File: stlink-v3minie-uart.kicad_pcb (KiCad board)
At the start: 2 copper layers, 10 x 3 mm, 3 parts, among them J1 Conn_01x05, J2 Conn_02x05_Top_Bottom, J3 Conn_01x04_Pin

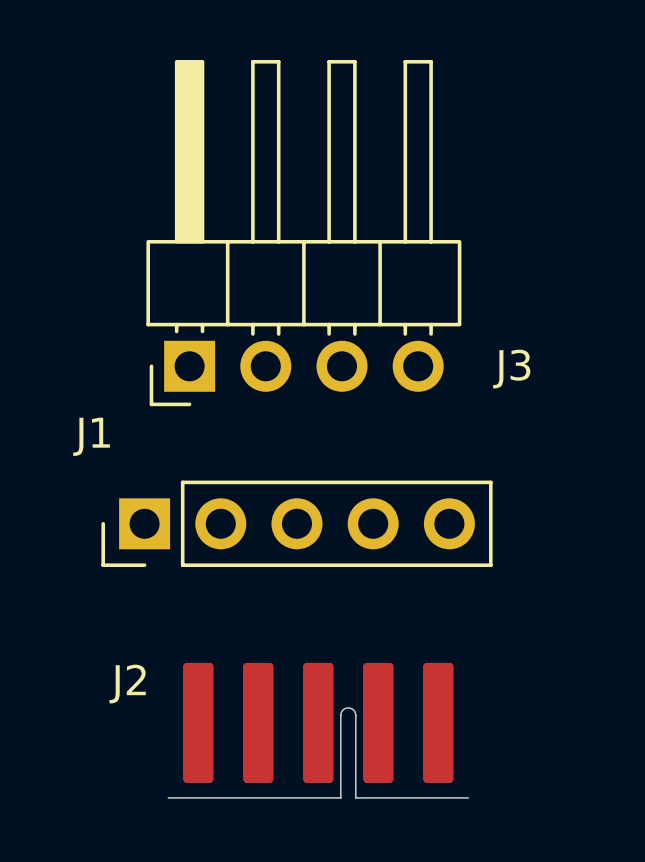
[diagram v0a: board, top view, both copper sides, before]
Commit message: pcb: oui
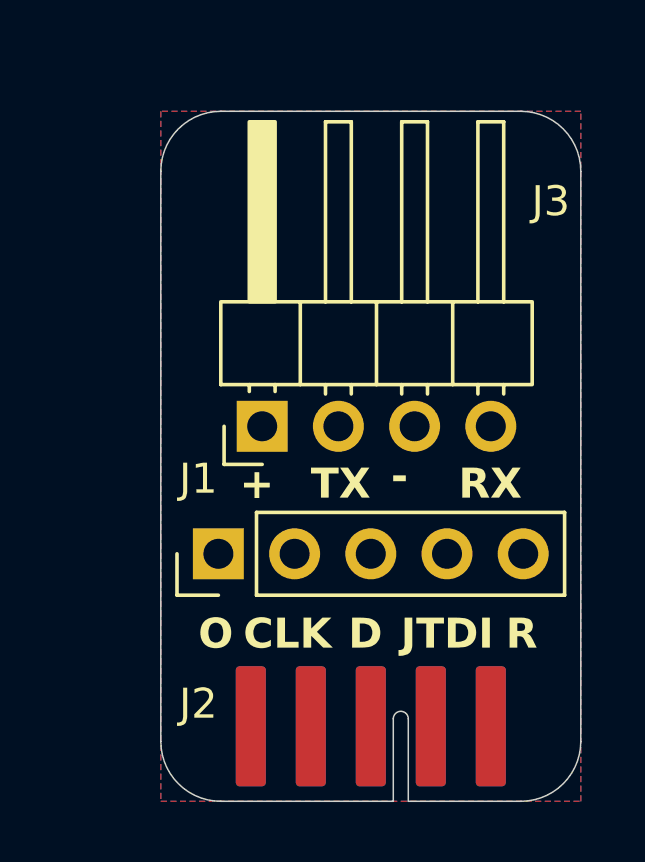
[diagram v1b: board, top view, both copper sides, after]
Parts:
- moved J3 3.14 mm to (146.4, 103.5)
- moved J1 2.66 mm to (144.9, 107.8)
- moved J2 1.75 mm to (147.0, 116.0)
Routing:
- added copper zone on B.Cu, net GND
- added copper zone on F.Cu, net GND
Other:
- board size 10 x 3 mm -> 14 x 23 mm
- board text added: "+"
- board text added: "-"
- board text added: "CLK"
- board text added: "D"
- board text added: "JTDI"
- board text added: "O"
- board text added: "R"
- board text added: "RX"
- board text added: "TX"
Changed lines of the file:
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@@
 	(footprint "GLCS:KYOCERA_AVX9159-006"
 		(layer "F.Cu")
-		(at 145.25 115.8875 180)
+		(at 147 116 180)
 		(descr "board to board 10 pin edge connector https://www.kyocera-avx.com/download/connectors/Conn-Sales-Drawings/9XXX/9159-06X.zip")
 		(tags "edge b2b")
 		(property "Reference" "J2"
-			(at 3.25 3.8875 0)
+			(at 2.75 3.25 0)
 			(layer "F.SilkS")
 			(effects
@@
 	(footprint "Connector_PinHeader_2.54mm:PinHeader_1x05_P2.54mm_Vertical"
 		(layer "F.Cu")
-		(at 142.46 106.75 90)
+		(at 144.92 107.75 90)
 		(descr "Through hole straight pin header, 1x05, 2.54mm pitch, single row")
 		(tags "Through hole pin header THT 1x05 2.54mm single row")
 		(property "Reference" "J1"
-			(at 3 -1.67 180)
+			(at 2.5 -0.67 180)
 			(layer "F.SilkS")
 			(effects
@@
 	(footprint "Connector_PinHeader_2.54mm:PinHeader_1x04_P2.54mm_Horizontal"
 		(layer "F.Cu")
-		(at 143.96 101.5 90)
+		(at 146.38 103.5 90)
 		(descr "Through hole angled pin header, 1x04, 2.54mm pitch, 6mm pin length, single row")
 		(tags "Through hole angled pin header THT 1x04 2.54mm single row")
 		(property "Reference" "J3"
-			(at 0 10.83 180)
+			(at 7.5 9.62 180)
 			(layer "F.SilkS")
 			(effects
@@
 			)
 		)
+	)
+	(gr_arc
+		(start 143 95)
+		(mid 143.585786 93.585786)
+		(end 145 93)
+		(stroke
+			(width 0.05)
+			(type default)
+		)
+		(layer "Edge.Cuts")
+	)
+	(gr_line
+		(start 143 114)
+		(end 143 95)
+		(stroke
+			(width 0.05)
+			(type default)
+		)
+		(layer "Edge.Cuts")
+	)
+	(gr_arc
+		(start 145 116)
+		(mid 143.585786 115.414214)
+		(end 143 114)
+		(stroke
+			(width 0.05)
+			(type default)
+		)
+		(layer "Edge.Cuts")
+	)
+	(gr_line
+		(start 155 93)
+		(end 145 93)
+		(stroke
+			(width 0.05)
+			(type default)
+		)
+		(layer "Edge.Cuts")
+	)
+	(gr_arc
+		(start 155 93)
+		(mid 156.414214 93.585786)
+		(end 157 95)
+		(stroke
+			(width 0.05)
+			(type default)
+		)
+		(layer "Edge.Cuts")
+	)
+	(gr_arc
+		(start 157 114)
+		(mid 156.414214 115.414214)
+		(end 155 116)
+		(stroke
+			(width 0.05)
+			(type default)
+		)
+		(layer "Edge.Cuts")
+	)
+	(gr_line
+		(start 157 114)
+		(end 157 95)
+		(stroke
+			(width 0.05)
+			(type default)
+		)
+		(layer "Edge.Cuts")
+	)
+	(gr_text "O"
+		(at 144.25 111 0)
+		(layer "F.SilkS" knockout)
+		(effects
+			(font
+				(size 1 1)
+				(thickness 0.2)
+				(bold yes)
+			)
+			(justify left bottom)
+		)
+	)
+	(gr_text "+"
+		(at 145.628589 106.012058 0)
+		(layer "F.SilkS" knockout)
+		(effects
+			(font
+				(size 1 1)
+				(thickness 0.2)
+				(bold yes)
+			)
+			(justify left bottom)
+		)
+	)
+	(gr_text "CLK"
+		(at 145.75 111 0)
+		(layer "F.SilkS" knockout)
+		(effects
+			(font
+				(size 1 1)
+				(thickness 0.2)
+				(bold yes)
+			)
+			(justify left bottom)
+		)
+	)
+	(gr_text "TX"
+		(at 148 106 0)
+		(layer "F.SilkS" knockout)
+		(effects
+			(font
+				(size 1 1)
+				(thickness 0.2)
+				(bold yes)
+			)
+			(justify left bottom)
+		)
+	)
+	(gr_text "D"
+		(at 149.25 111 0)
+		(layer "F.SilkS" knockout)
+		(effects
+			(font
+				(size 1 1)
+				(thickness 0.2)
+				(bold yes)
+			)
+			(justify left bottom)
+		)
+	)
+	(gr_text "-"
+		(at 150.67177 105.750075 0)
+		(layer "F.SilkS" knockout)
+		(effects
+			(font
+				(size 1 1)
+				(thickness 0.2)
+				(bold yes)
+			)
+			(justify left bottom)
+		)
+	)
+	(gr_text "JTDI"
+		(at 151 111 0)
+		(layer "F.SilkS" knockout)
+		(effects
+			(font
+				(size 1 1)
+				(thickness 0.2)
+				(bold yes)
+			)
+			(justify left bottom)
+		)
+	)
+	(gr_text "RX"
+		(at 152.922445 106.00015 0)
+		(layer "F.SilkS" knockout)
+		(effects
+			(font
+				(size 1 1)
+				(thickness 0.2)
+				(bold yes)
+			)
+			(justify left bottom)
+		)
+	)
+	(gr_text "R"
+		(at 154.5 111 0)
+		(layer "F.SilkS" knockout)
+		(effects
+			(font
+				(size 1 1)
+				(thickness 0.2)
+				(bold yes)
+			)
+			(justify left bottom)
+		)
+	)
+	(zone
+		(net "GND")
+		(layers "F.Cu" "B.Cu")
+		(hatch edge 0.5)
+		(connect_pads
+			(clearance 0.2)
+		)
+		(min_thickness 0.15)
+		(fill yes
+			(thermal_gap 0.35)
+			(thermal_bridge_width 0.35)
+			(island_removal_mode 0)
+		)
+		(polygon
+			(pts
+				(xy 143 93) (xy 143 116) (xy 157 116) (xy 157 93)
+			)
+		)
